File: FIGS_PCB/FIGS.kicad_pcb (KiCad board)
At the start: 2 copper layers, 54.1 x 52.8 mm, 66 parts, among them IC1 CY8C4245AXI-483, J1 CAPSENSE_CON, J10 HAPTIC_M, J2 FINGCONN, J3 BLUTH, J4 IMU, J5 SERVO_0, J6 SERVO_1, J7 SERVO_2, J8 PROGRAMMER, J9 SERVO_3, Q1 FDV303N, Q2 FDV303N, Q3 FDV303N, Q4 FDV303N, Q5 FDV303N, SW1 SW_ON, SW2 SW_Push, U1 TLV1117-33

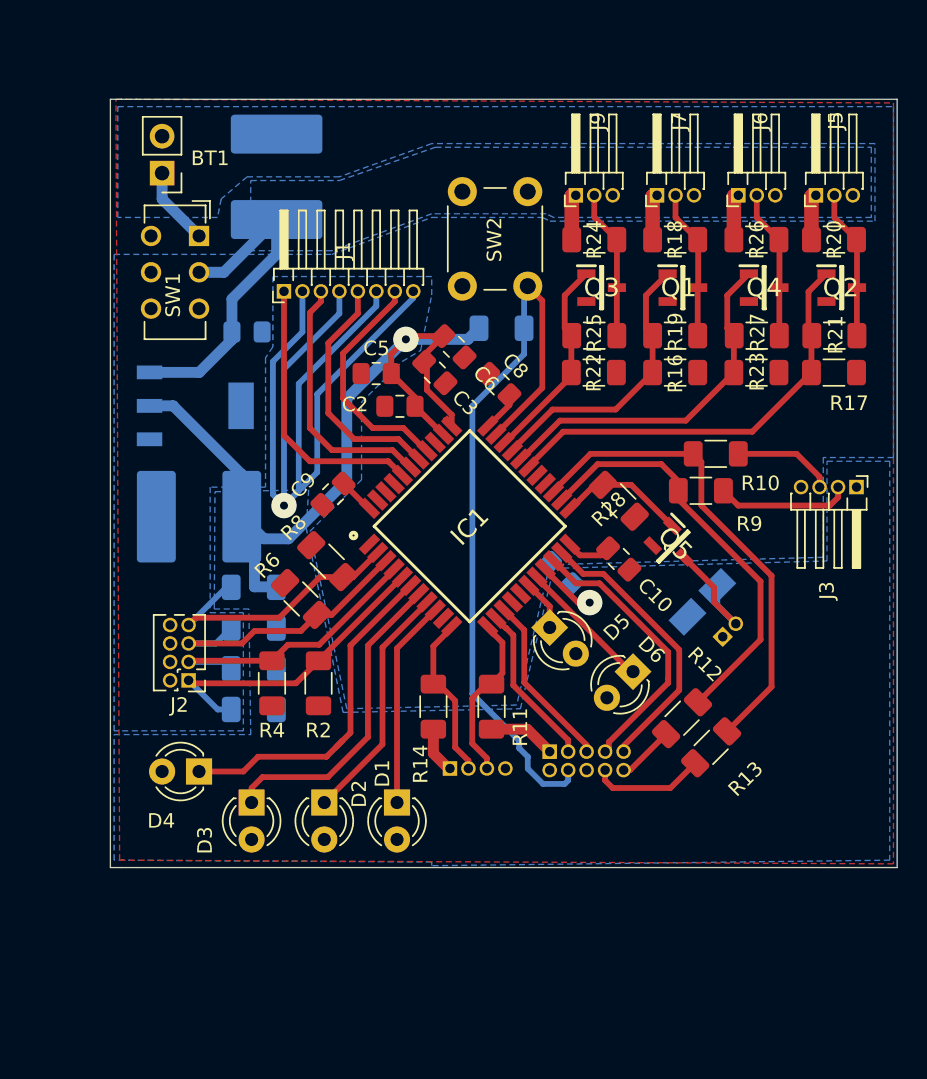
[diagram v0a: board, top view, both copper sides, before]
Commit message: PCB changed
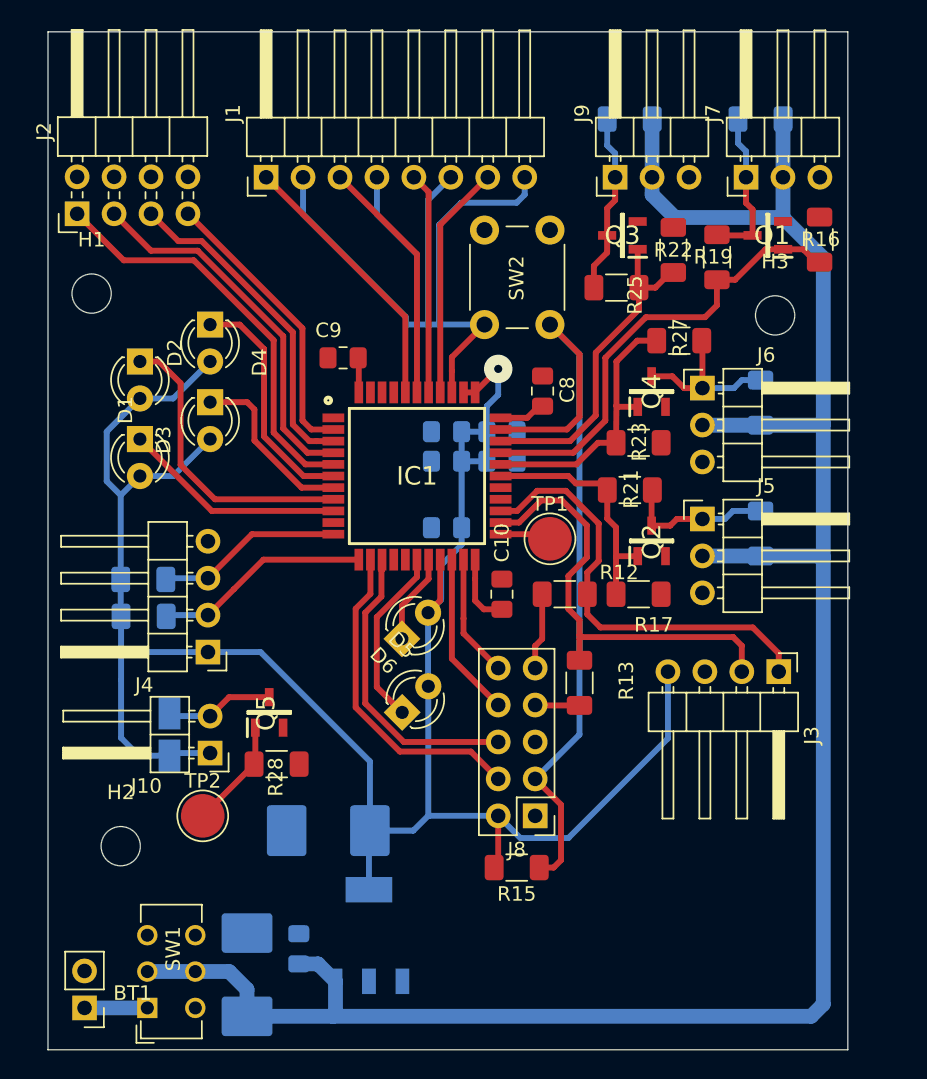
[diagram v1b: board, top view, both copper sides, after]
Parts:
- removed R1, R3, R5, R7: 5.6k, Resistor_SMD:R_1206_3216Metric_Pad1.30x1.75mm_HandSolder
- removed R10, R9: 0, Resistor_SMD:R_1206_3216Metric_Pad1.30x1.75mm_HandSolder
- removed R2, R4, R6, R8: nc, Resistor_SMD:R_1206_3216Metric_Pad1.30x1.75mm_HandSolder
- added H1: MountingHole, MountingHole:MountingHole_2.7mm, F.Cu at (33.0, 38.0)
- added H2: MountingHole, MountingHole:MountingHole_2.7mm, F.Cu at (35.0, 76.0)
- added H3: MountingHole, MountingHole:MountingHole_2.7mm, F.Cu at (80.0, 39.5)
- added TP1: TestPoint, TestPoint:TestPoint_Pad_D3.0mm, F.Cu at (64.5, 54.9)
- added TP2: TestPoint, TestPoint:TestPoint_Pad_D3.0mm, F.Cu at (40.6, 73.9)
- C11, C4: footprint Capacitor_Tantalum_SMD:CP_EIA-7260-28_AVX-M_Pad2.68x6.30mm_HandSolder -> Capacitor_Tantalum_SMD:CP_EIA-7132-20_AVX-U_Pad2.72x3.50mm_HandSolder
- C2, C3, C5, C6, R11, R14, R18, R20, R24, R26: moved to B.Cu
- J1: footprint Connector_PinHeader_1.27mm:PinHeader_1x08_P1.27mm_Horizontal -> Connector_PinHeader_2.54mm:PinHeader_1x08_P2.54mm_Horizontal
- J10: footprint Connector_PinHeader_1.27mm:PinHeader_1x02_P1.27mm_Horizontal -> Connector_PinHeader_2.54mm:PinHeader_1x02_P2.54mm_Horizontal; moved to F.Cu
- J2: footprint Connector_PinHeader_1.27mm:PinHeader_2x04_P1.27mm_Vertical -> Connector_PinHeader_2.54mm:PinHeader_2x04_P2.54mm_Horizontal
- J3: footprint Connector_PinHeader_1.27mm:PinHeader_1x04_P1.27mm_Horizontal -> Connector_PinHeader_2.54mm:PinHeader_1x04_P2.54mm_Horizontal
- J4: footprint Connector_PinHeader_1.27mm:PinHeader_1x04_P1.27mm_Horizontal -> Connector_PinHeader_2.54mm:PinHeader_1x04_P2.54mm_Horizontal; moved to F.Cu
- J5, J6, J7, J9: footprint Connector_PinHeader_1.27mm:PinHeader_1x03_P1.27mm_Horizontal -> Connector_PinHeader_2.54mm:PinHeader_1x03_P2.54mm_Horizontal
- J8: footprint Connector_PinHeader_1.27mm:PinHeader_2x05_P1.27mm_Horizontal -> Connector_PinHeader_2.54mm:PinHeader_2x05_P2.54mm_Vertical; moved to F.Cu
- R15: moved to F.Cu
- moved BT1 57.7 mm to (32.5, 87.1)
- moved C4 54.9 mm to (43.7, 84.8)
- moved SW1 53.2 mm to (36.8, 87.1), turned to 90 degrees
- moved C7 42.6 mm to (47.2, 83.1), turned to 90 degrees
- moved U1 38.3 mm to (52.1, 82.1), turned to 90 degrees
- moved D7 37.8 mm to (38.4, 68.3), turned to 90 degrees
- moved R15 37.1 mm to (62.2, 77.5)
- moved J10 36.1 mm to (41.1, 69.6), turned to 180 degrees
- moved J2 33.0 mm to (32.0, 32.5), turned to 90 degrees
- moved D2 32.9 mm to (36.3, 42.7)
- moved D4 30.7 mm to (41.1, 40.1), turned to 270 degrees
- moved D1 30.6 mm to (36.3, 48.0)
- moved Q5 30.0 mm to (45.2, 66.8), turned to 90 degrees
- moved R28 29.7 mm to (45.7, 70.4), turned to 180 degrees
- moved D3 27.7 mm to (41.1, 45.5)
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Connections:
- IC1 pad 24: /Rx_1 -> /BT_UART_TX
- IC1 pad 25: /Tx_1 -> /BT_UART_RX
- J3 pad 1: +3V3 -> /BT_UART_RX
- J3 pad 3: /BT_UART_RX -> GNDA
- J3 pad 4: GNDA -> +3V3
- J4 pad 2: /IMU_SCL -> /IMU_SDA
- J4 pad 3: /IMU_SDA -> /IMU_SCL
- J5 pad 1: +BATT -> /CTRLS0
- J5 pad 2: /CTRLS0 -> +BATT
- J6 pad 1: +BATT -> /CTRLS1
- J6 pad 2: /CTRLS1 -> +BATT
- J7 pad 1: +BATT -> /CTRLS2
- J7 pad 2: /CTRLS2 -> +BATT
- J8 pad 1: +3V3 -> GNDA
- J8 pad 10: /KP_TX -> /TUNER_SDA
- J8 pad 2: GNDA -> +3V3
- J8 pad 3: /SWD_IO -> /XRES
- J8 pad 4: /XRES -> /SWD_IO
- J8 pad 5: /SWD_CLK -> Net-(J8-Pad5)
- J8 pad 6: Net-(J8-Pad6) -> /SWD_CLK
- J8 pad 7: /TUNER_SCL -> /KP_TX
- J8 pad 8: /KP_RX -> /TUNER_SCL
- J8 pad 9: /TUNER_SDA -> /KP_RX
- J9 pad 1: +BATT -> /CTRLS3
- J9 pad 2: /CTRLS3 -> +BATT
- R11 pad 2: /IMU_SDA -> /IMU_SCL
- R12 pad 1: /Rx_1 -> /BT_UART_RX
- R12 pad 2: /KP_TX -> /KP_RX
- R13 pad 1: /KP_RX -> /KP_TX
- R13 pad 2: /Tx_1 -> /BT_UART_TX
- R14 pad 2: /IMU_SCL -> /IMU_SDA
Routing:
- net +BATT: track 35.3 -> 148.3 mm
- net +3V3: track 75.2 -> 151.4 mm, vias 2 -> 1
- net /Tx_1: track 33.8 -> 0.00 mm
- net /Rx_1: track 28.9 -> 0.00 mm
- net /BT_UART_RX: track 7.16 -> 30.4 mm
- net /BT_UART_TX: track 9.24 -> 30.7 mm
- net /SERVOS_OUT0: track 29.6 -> 17.1 mm
- net /SERVOS_OUT2: track 19.5 -> 31.7 mm
- net /SWD_IO: track 11.2 -> 22.4 mm
- net /TUNER_SDA: track 19.5 -> 8.45 mm
- net /SERVOS_LED1: track 21.8 -> 12.2 mm
- net /STATUS_LED1: track 3.49 -> 12.4 mm
- net /SWD_CLK: track 12.0 -> 20.6 mm
- net /SERVOS_OUT3: track 14.4 -> 22.8 mm
- net /TUNER_SCL: track 19.1 -> 11.3 mm
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- removed copper zone on B.Cu, net +3V3
- removed copper zone on B.Cu, net +BATT
- removed copper zone on B.Cu, net GNDA
- removed copper zone on F.Cu, net GNDA
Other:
- board size 54.1 x 52.8 mm -> 55 x 70 mm
- net class Default: clearance 0.25 -> 0.254; trace_width 0.4 -> 0.4064; via_dia 1.75 -> 1.9558; via_drill 0.55 -> 0.5588
- net class ThickPower: clearance 0.5 -> 0.254; trace_width 0.75 -> 1.016; via_dia 1.75 -> 1.9558; via_drill 0.55 -> 0.5588
- rule trace_clearance: 0.25 -> 0.254
